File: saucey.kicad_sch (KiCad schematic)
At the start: 48 parts, among them J1 Conn_01x02_Socket, J2 USB_C_Receptacle_USB2.0_16P, M1 Motor_DC, M2 Motor_DC, M3 Motor_DC, M4 Motor_DC, Q1 AO3401A, Q3 SI2306, Q4 SI2306, Q5 SI2306, Q6 SI2306, SW1 SW_Push, SW2 SW_Push, U1 ESP32-S3-WROOM-1, U2 AMS1117-3.3, U4 MPU-6050

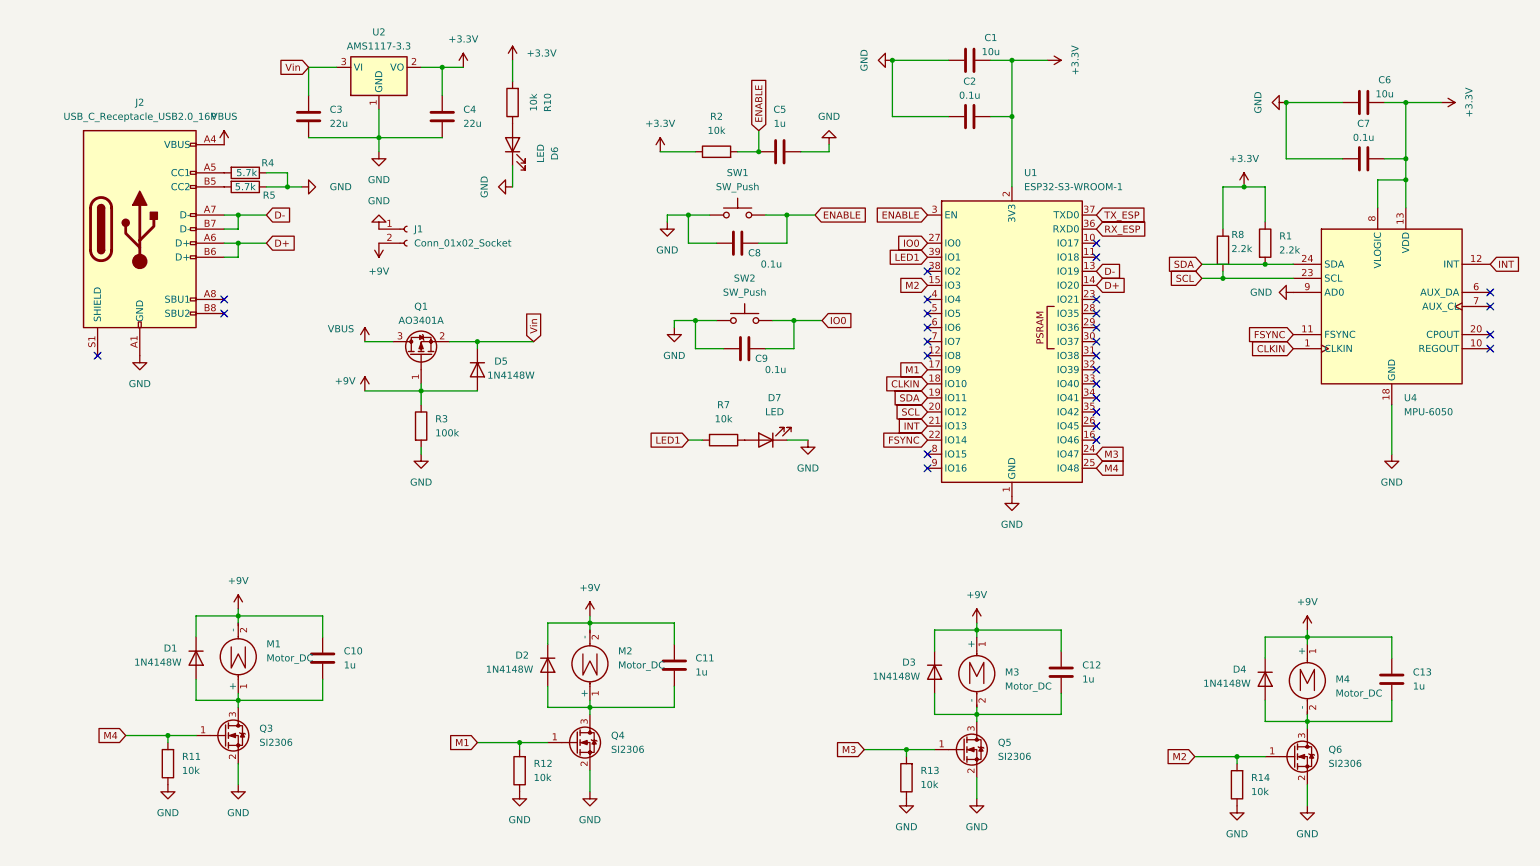
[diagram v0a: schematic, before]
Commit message: Add files via upload
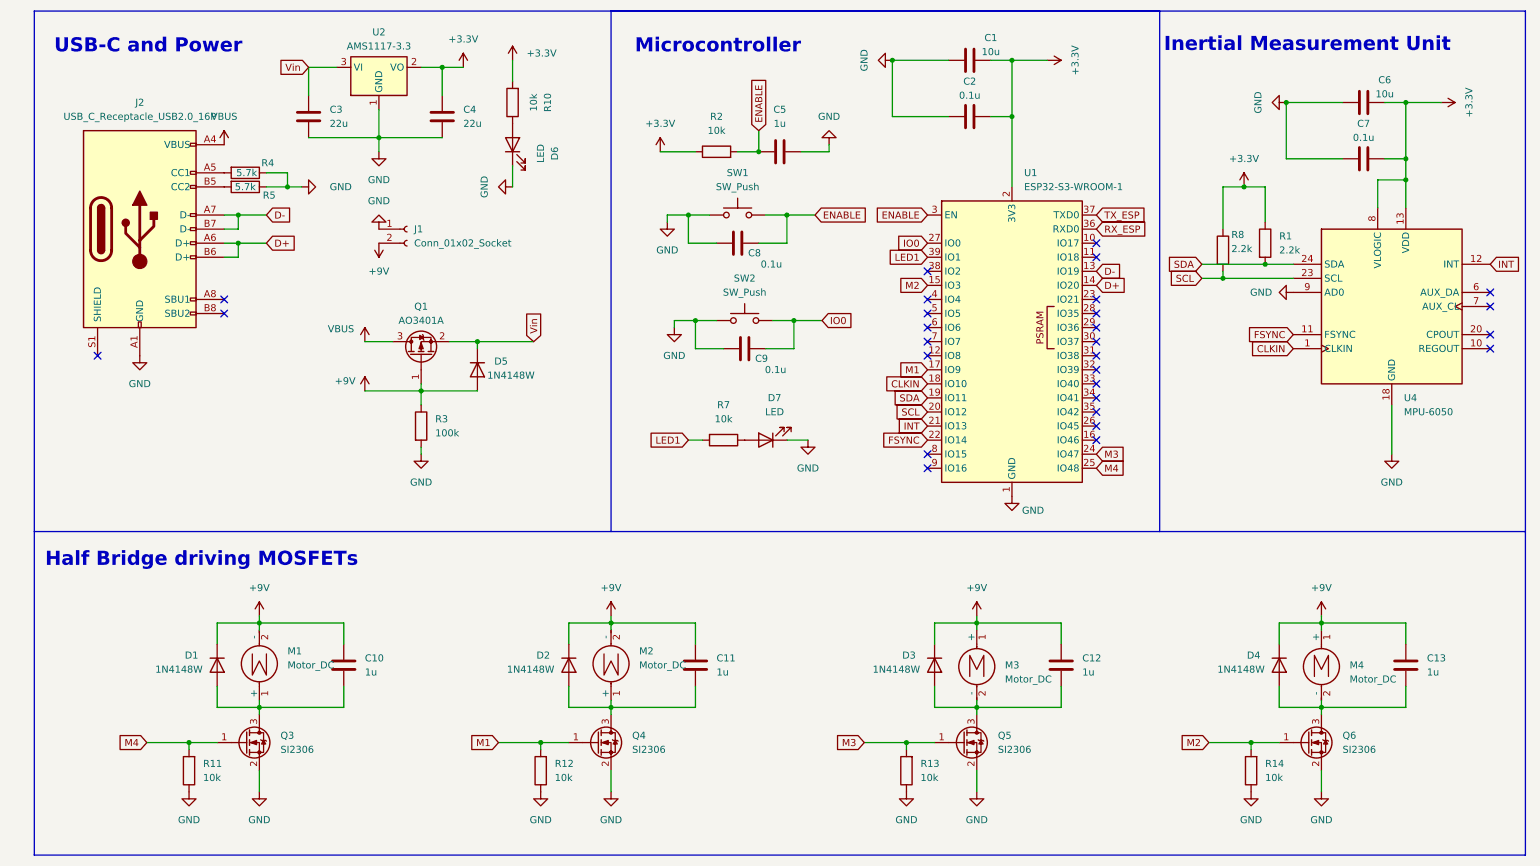
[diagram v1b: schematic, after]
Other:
- note added: "Half Bridge driving MOSFETs"
- note added: "Inertial Measurement Unit"
- note added: "Microcontroller"
- note added: "USB-C and Power"
- moved on the sheet: C10, C11, C12, C13, D1, D2, D3, D4, M1, M2, M3, M4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
